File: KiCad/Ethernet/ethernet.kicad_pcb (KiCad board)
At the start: 2 copper layers, 100 x 100 mm, 32 parts, among them IC1 74LS32, IC2 74LS688, IC3 74LVC245, IC4 74LVC245, IC5 74LVC245, J1 NKC-Bus, J2 Jumper, J3 Conn_01x09, J5 SBHE_Jumper, J6 A0_Jumper, Q1 BC547, Q2 BC557, SW1 SW_DIP_x04, U1 LT1086-3.3

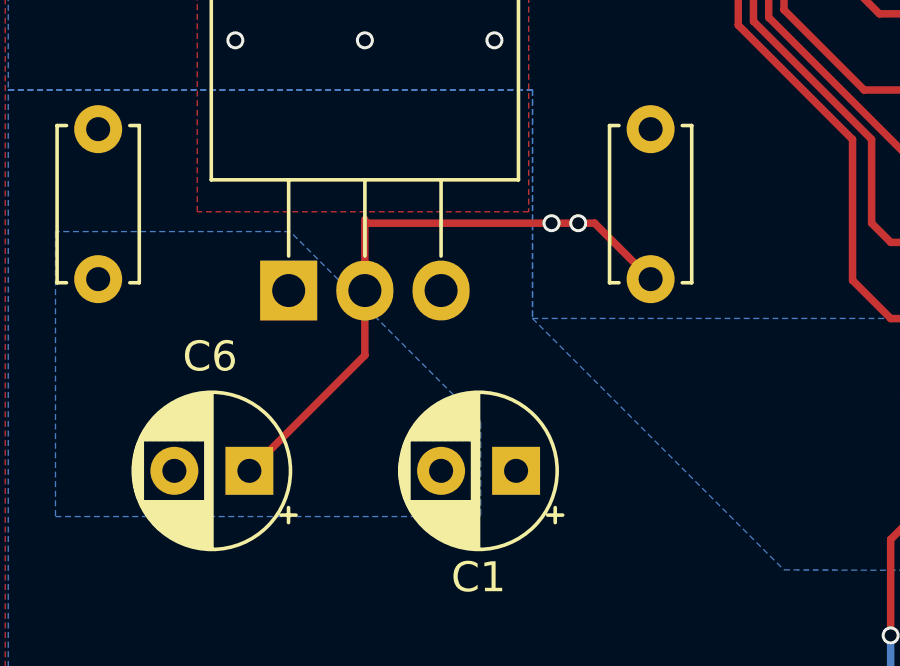
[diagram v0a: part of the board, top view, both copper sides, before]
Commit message: minor bugfix
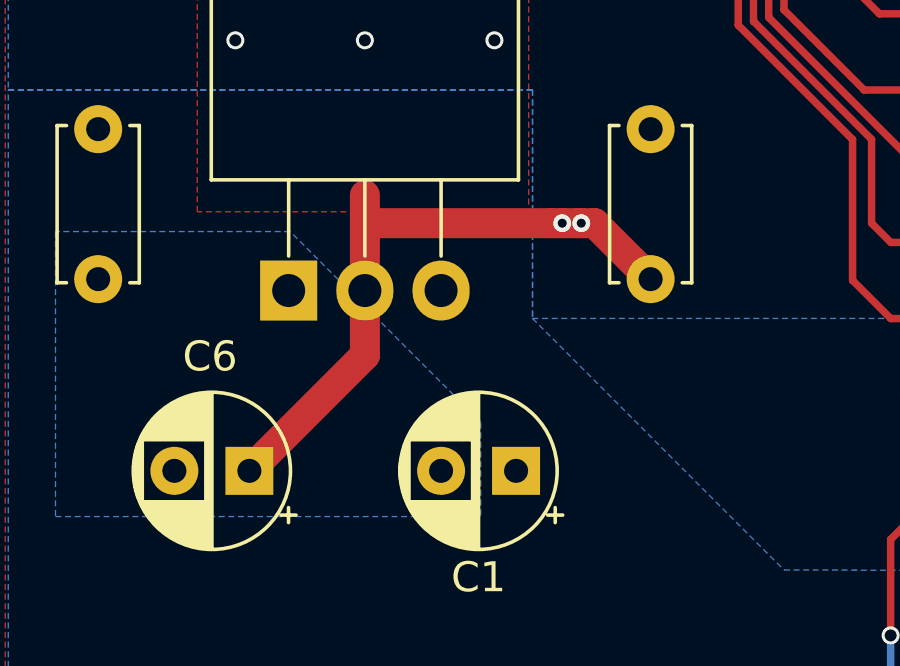
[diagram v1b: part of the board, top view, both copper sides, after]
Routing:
- net +3V3: track 20.1 -> 21.0 mm
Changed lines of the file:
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@@
   (segment (start 90.17 124.714) (end 90.678 125.222) (width 0.25) (layer "B.Cu") (net 2))
   (segment (start 90.17 120.65) (end 90.17 124.714) (width 0.25) (layer "B.Cu") (net 2))
-  (segment (start 49.53 122.26) (end 49.53 124.42) (width 0.25) (layer "F.Cu") (net 3))
-  (segment (start 56.642 120.015) (end 57.19 120.015) (width 0.25) (layer "F.Cu") (net 3))
-  (segment (start 55.753 120.015) (end 56.642 120.015) (width 0.25) (layer "F.Cu") (net 3))
-  (segment (start 49.657 120.015) (end 55.753 120.015) (width 0.25) (layer "F.Cu") (net 3))
-  (segment (start 49.53 122.26) (end 49.53 119.888) (width 0.25) (layer "F.Cu") (net 3))
-  (segment (start 57.19 120.015) (end 59.055 121.88) (width 0.25) (layer "F.Cu") (net 3))
-  (segment (start 49.53 124.42) (end 45.68 128.27) (width 0.25) (layer "F.Cu") (net 3))
+  (segment (start 49.53 122.26) (end 49.53 124.42) (width 1) (layer "F.Cu") (net 3))
+  (segment (start 56.642 120.015) (end 56.7436 120.015) (width 1) (layer "F.Cu") (net 3))
+  (segment (start 49.53 122.26) (end 49.53 119.0752) (width 1) (layer "F.Cu") (net 3))
+  (segment (start 55.753 120.015) (end 56.1086 120.015) (width 1) (layer "F.Cu") (net 3))
+  (segment (start 56.1086 120.015) (end 56.642 120.015) (width 1) (layer "F.Cu") (net 3))
+  (segment (start 49.657 120.015) (end 55.753 120.015) (width 1) (layer "F.Cu") (net 3))
+  (segment (start 57.19 120.015) (end 59.055 121.88) (width 1) (layer "F.Cu") (net 3))
+  (segment (start 56.7436 120.015) (end 57.19 120.015) (width 1) (layer "F.Cu") (net 3))
+  (segment (start 49.53 124.42) (end 45.68 128.27) (width 1) (layer "F.Cu") (net 3))
   (via (at 45.212 109.982) (size 0.6) (drill 0.4) (layers "F.Cu" "B.Cu") (free) (net 3))
   (via (at 45.212 107.95) (size 0.6) (drill 0.4) (layers "F.Cu" "B.Cu") (free) (net 3))
@@
   (via (at 53.848 112.014) (size 0.6) (drill 0.4) (layers "F.Cu" "B.Cu") (free) (net 3))
   (via (at 53.848 105.664) (size 0.6) (drill 0.4) (layers "F.Cu" "B.Cu") (free) (net 3))
-  (via (at 56.642 120.015) (size 0.6) (drill 0.4) (layers "F.Cu" "B.Cu") (net 3))
   (via (at 49.53 113.919) (size 0.6) (drill 0.4) (layers "F.Cu" "B.Cu") (free) (net 3))
   (via (at 45.212 112.014) (size 0.6) (drill 0.4) (layers "F.Cu" "B.Cu") (free) (net 3))
   (via (at 53.848 103.505) (size 0.6) (drill 0.4) (layers "F.Cu" "B.Cu") (free) (net 3))
   (via (at 49.53 110.109) (size 0.6) (drill 0.4) (layers "F.Cu" "B.Cu") (free) (net 3))
+  (via (at 56.7436 120.015) (size 0.6) (drill 0.3) (layers "F.Cu" "B.Cu") (net 3))
   (via (at 53.848 113.919) (size 0.6) (drill 0.4) (layers "F.Cu" "B.Cu") (free) (net 3))
   (via (at 53.848 107.823) (size 0.6) (drill 0.4) (layers "F.Cu" "B.Cu") (free) (net 3))
@@
   (via (at 53.848 110.109) (size 0.6) (drill 0.4) (layers "F.Cu" "B.Cu") (free) (net 3))
   (via (at 45.212 103.505) (size 0.6) (drill 0.4) (layers "F.Cu" "B.Cu") (free) (net 3))
+  (via (at 56.1086 120.015) (size 0.6) (drill 0.3) (layers "F.Cu" "B.Cu") (net 3))
   (via (at 45.212 105.537) (size 0.6) (drill 0.4) (layers "F.Cu" "B.Cu") (free) (net 3))
-  (via (at 55.753 120.015) (size 0.6) (drill 0.4) (layers "F.Cu" "B.Cu") (net 3))
   (segment (start 99.380411 137.703189) (end 96.266 140.8176) (width 0.25) (layer "F.Cu") (net 4))
   (segment (start 96.266 147.32) (end 98.176 149.23) (width 0.25) (layer "F.Cu") (net 4))
